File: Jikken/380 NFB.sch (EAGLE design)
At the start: 6 parts

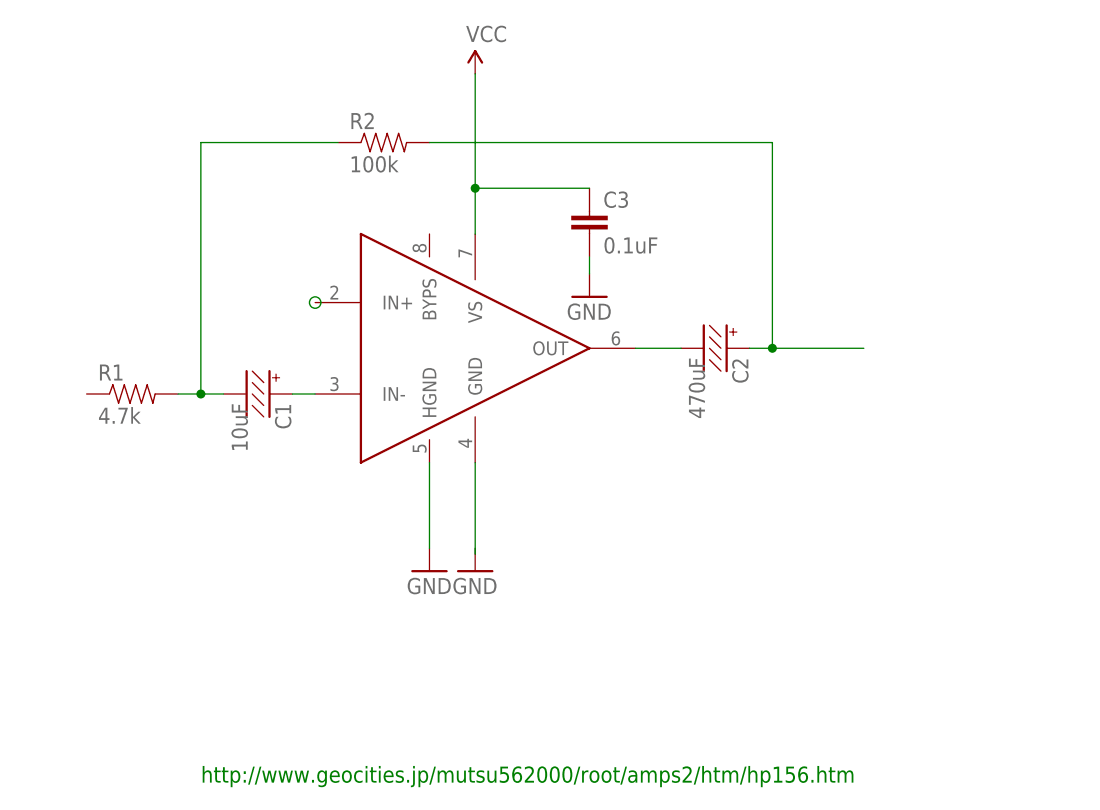
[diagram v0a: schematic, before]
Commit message: lm380
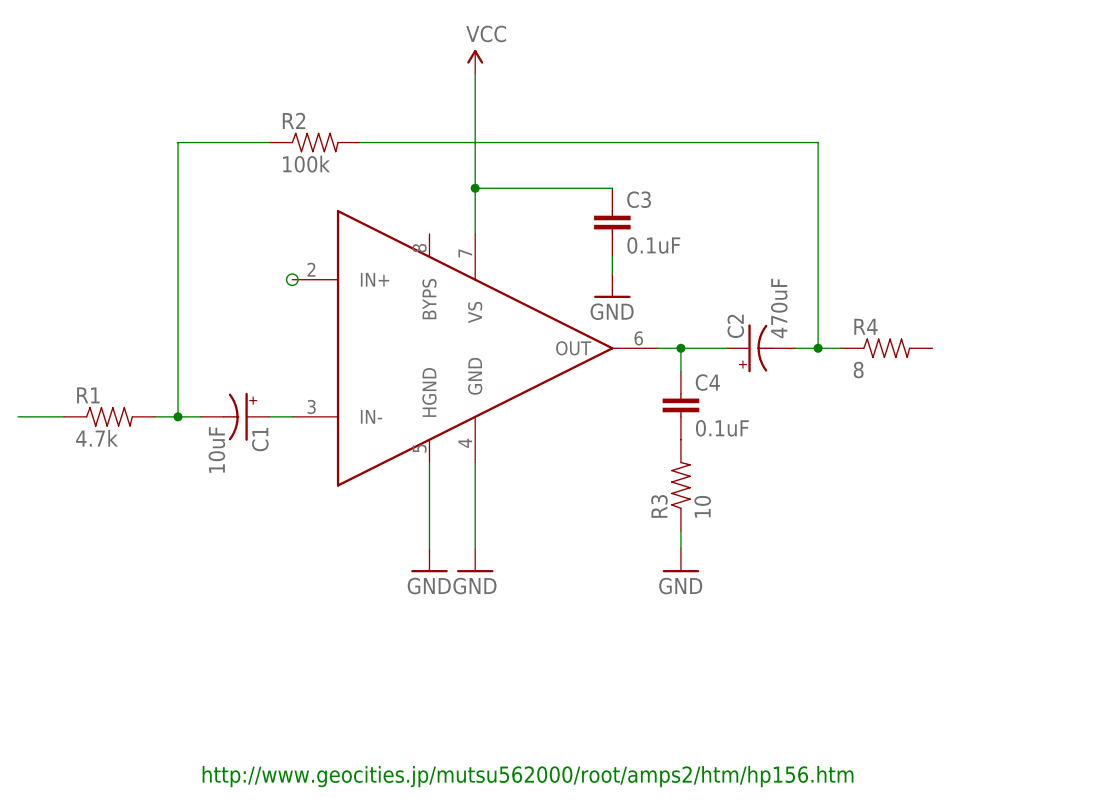
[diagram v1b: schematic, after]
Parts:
- added C4: 0.1uF, SparkFun:CAPKIT
- added R3: 10, My Library:RESISTORAXIAL-0.3
- added R4: 8, My Library:RESISTORAXIAL-0.3
- C1: device My Library:CAP_POLPTH2 -> SparkFun:CAP_POLPTH1
- C2: device My Library:CAP_POLPTH2 -> SparkFun:CAP_POLPTH4
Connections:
- removed net N$6: U$1.GND
- new net N$5: C4.2, R3.2
- new net N$7: R1.1
- net GND: now also R3.1, U$1.GND, U$1.HGND
- net N$3: now also C2.-, R4.1; no longer C2.+
- net N$4: now also C2.+, C4.1; no longer C2.-
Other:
- moved on the sheet: C3, R1, R2
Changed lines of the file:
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@@
 <part name="U$1" library="My Library" deviceset="LM380" device="N-8"/>
 <part name="R1" library="My Library" deviceset="RESISTOR" device="AXIAL-0.3" value="4.7k"/>
-<part name="C1" library="My Library" deviceset="CAP_POL" device="PTH2" value="10uF"/>
-<part name="C2" library="My Library" deviceset="CAP_POL" device="PTH2" value="470uF"/>
+<part name="C1" library="SparkFun" deviceset="CAP_POL" device="PTH1" value="10uF"/>
+<part name="C2" library="SparkFun" deviceset="CAP_POL" device="PTH4" value="470uF"/>
 <part name="R2" library="My Library" deviceset="RESISTOR" device="AXIAL-0.3" value="100k"/>
 <part name="P+1" library="SparkFun" deviceset="VCC" device=""/>
@@
 <part name="C3" library="SparkFun" deviceset="CAP" device="KIT" value="0.1uF"/>
 <part name="GND3" library="SparkFun" deviceset="GND" device=""/>
+<part name="R3" library="My Library" deviceset="RESISTOR" device="AXIAL-0.3" value="10"/>
+<part name="C4" library="SparkFun" deviceset="CAP" device="KIT" value="0.1uF"/>
+<part name="GND4" library="SparkFun" deviceset="GND" device=""/>
+<part name="R4" library="My Library" deviceset="RESISTOR" device="AXIAL-0.3" value="8"/>
 </parts>
 <sheets>
@@
 <plain>
 <text x="48.26" y="7.62" size="1.778" layer="91">http://www.geocities.jp/mutsu562000/root/amps2/htm/hp156.htm</text>
-<circle x="60.96" y="60.96" radius="0.635" width="0.1524" layer="91"/>
+<circle x="58.42" y="63.5" radius="0.635" width="0.1524" layer="91"/>
 </plain>
 <instances>
-<instance part="U$1" gate="G$1" x="76.2" y="55.88"/>
-<instance part="R1" gate="G$1" x="40.64" y="50.8"/>
-<instance part="C1" gate="G$1" x="55.88" y="50.8" rot="R270"/>
-<instance part="C2" gate="G$1" x="106.68" y="55.88" rot="R270"/>
-<instance part="R2" gate="G$1" x="68.58" y="78.74"/>
+<instance part="U$1" gate="G$1" x="78.74" y="55.88"/>
+<instance part="R1" gate="G$1" x="38.1" y="48.26"/>
+<instance part="C1" gate="G$1" x="53.34" y="48.26" rot="R270"/>
+<instance part="C2" gate="G$1" x="109.22" y="55.88" rot="R90"/>
+<instance part="R2" gate="G$1" x="60.96" y="78.74"/>
 <instance part="P+1" gate="1" x="78.74" y="86.36"/>
 <instance part="GND1" gate="1" x="78.74" y="31.115"/>
-<instance part="GND2" gate="1" x="91.44" y="61.595"/>
-<instance part="C3" gate="G$1" x="91.44" y="68.58"/>
+<instance part="GND2" gate="1" x="93.98" y="61.595"/>
+<instance part="C3" gate="G$1" x="93.98" y="68.58"/>
 <instance part="GND3" gate="1" x="73.66" y="31.115"/>
+<instance part="R3" gate="G$1" x="101.6" y="40.64" rot="R90"/>
+<instance part="C4" gate="G$1" x="101.6" y="48.26"/>
+<instance part="GND4" gate="1" x="101.6" y="31.115"/>
+<instance part="R4" gate="G$1" x="124.46" y="55.88"/>
 </instances>
 <busses>
@@
 <pinref part="C1" gate="G$1" pin="-"/>
 <pinref part="R1" gate="G$1" pin="2"/>
-<wire x1="50.8" y1="50.8" x2="48.26" y2="50.8" width="0.1524" layer="91"/>
+<wire x1="48.26" y1="48.26" x2="45.72" y2="48.26" width="0.1524" layer="91"/>
 <pinref part="R2" gate="G$1" pin="1"/>
-<wire x1="48.26" y1="50.8" x2="45.72" y2="50.8" width="0.1524" layer="91"/>
-<wire x1="63.5" y1="78.74" x2="48.26" y2="78.74" width="0.1524" layer="91"/>
-<wire x1="48.26" y1="78.74" x2="48.26" y2="50.8" width="0.1524" layer="91"/>
-<junction x="48.26" y="50.8"/>
+<wire x1="45.72" y1="48.26" x2="43.18" y2="48.26" width="0.1524" layer="91"/>
+<wire x1="55.88" y1="78.74" x2="45.72" y2="78.74" width="0.1524" layer="91"/>
+<wire x1="45.72" y1="78.74" x2="45.72" y2="48.26" width="0.1524" layer="91"/>
+<junction x="45.72" y="48.26"/>
 </segment>
 </net>
 <net name="N$3" class="0">
 <segment>
-<pinref part="C2" gate="G$1" pin="+"/>
-<wire x1="109.22" y1="55.88" x2="111.76" y2="55.88" width="0.1524" layer="91"/>
-<wire x1="111.76" y1="55.88" x2="121.92" y2="55.88" width="0.1524" layer="91"/>
-<wire x1="111.76" y1="55.88" x2="111.76" y2="78.74" width="0.1524" layer="91"/>
+<wire x1="116.84" y1="55.88" x2="119.38" y2="55.88" width="0.1524" layer="91"/>
+<wire x1="116.84" y1="55.88" x2="116.84" y2="78.74" width="0.1524" layer="91"/>
 <pinref part="R2" gate="G$1" pin="2"/>
-<wire x1="111.76" y1="78.74" x2="73.66" y2="78.74" width="0.1524" layer="91"/>
-<junction x="111.76" y="55.88"/>
-</segment>
-</net>
-<net name="N$4" class="0">
-<segment>
-<pinref part="U$1" gate="G$1" pin="OUT"/>
+<wire x1="116.84" y1="78.74" x2="66.04" y2="78.74" width="0.1524" layer="91"/>
 <pinref part="C2" gate="G$1" pin="-"/>
-<wire x1="96.52" y1="55.88" x2="101.6" y2="55.88" width="0.1524" layer="91"/>
+<wire x1="114.3" y1="55.88" x2="116.84" y2="55.88" width="0.1524" layer="91"/>
+<junction x="116.84" y="55.88"/>
+<pinref part="R4" gate="G$1" pin="1"/>
 </segment>
 </net>
@@
 <wire x1="78.74" y1="86.36" x2="78.74" y2="73.66" width="0.1524" layer="91"/>
 <wire x1="78.74" y1="73.66" x2="78.74" y2="68.58" width="0.1524" layer="91"/>
-<wire x1="78.74" y1="73.66" x2="91.44" y2="73.66" width="0.1524" layer="91"/>
+<wire x1="78.74" y1="73.66" x2="93.98" y2="73.66" width="0.1524" layer="91"/>
 <pinref part="C3" gate="G$1" pin="1"/>
 <junction x="78.74" y="73.66"/>
@@
 <wire x1="73.66" y1="43.18" x2="73.66" y2="33.655" width="0.1524" layer="91"/>
 <pinref part="GND3" gate="1" pin="GND"/>
+<pinref part="U$1" gate="G$1" pin="HGND"/>
 </segment>
 <segment>
 <pinref part="C3" gate="G$1" pin="2"/>
 <pinref part="GND2" gate="1" pin="GND"/>
-<wire x1="91.44" y1="64.135" x2="91.44" y2="66.04" width="0.1524" layer="91"/>
+<wire x1="93.98" y1="64.135" x2="93.98" y2="66.04" width="0.1524" layer="91"/>
 </segment>
-</net>
-<net name="N$6" class="0">
+<segment>
+<pinref part="R3" gate="G$1" pin="1"/>
+<pinref part="GND4" gate="1" pin="GND"/>
+<wire x1="101.6" y1="33.655" x2="101.6" y2="35.56" width="0.1524" layer="91"/>
+</segment>
 <segment>
 <pinref part="U$1" gate="G$1" pin="GND"/>
-<wire x1="78.74" y1="43.18" x2="78.74" y2="33.02" width="0.1524" layer="91"/>
+<wire x1="78.74" y1="43.18" x2="78.74" y2="33.655" width="0.1524" layer="91"/>
+<pinref part="GND1" gate="1" pin="GND"/>
 </segment>
 </net>
@@
 <pinref part="C1" gate="G$1" pin="+"/>
 <pinref part="U$1" gate="G$1" pin="IN-"/>
-<wire x1="58.42" y1="50.8" x2="60.96" y2="50.8" width="0.1524" layer="91"/>
+<wire x1="55.88" y1="48.26" x2="58.42" y2="48.26" width="0.1524" layer="91"/>
 </segment>
 </net>
+<net name="N$4" class="0">
+<segment>
+<pinref part="U$1" gate="G$1" pin="OUT"/>
+<pinref part="C2" gate="G$1" pin="+"/>
+<wire x1="99.06" y1="55.88" x2="101.6" y2="55.88" width="0.1524" layer="91"/>
+<pinref part="C4" gate="G$1" pin="1"/>
+<wire x1="101.6" y1="55.88" x2="106.68" y2="55.88" width="0.1524" layer="91"/>
+<wire x1="101.6" y1="55.88" x2="101.6" y2="53.34" width="0.1524" layer="91"/>
+<junction x="101.6" y="55.88"/>
+</segment>
+</net>
+<net name="N$5" class="0">
+<segment>
+<pinref part="C4" gate="G$1" pin="2"/>
+<pinref part="R3" gate="G$1" pin="2"/>
+</segment>
+</net>
+<net name="N$7" class="0">
+<segment>
+<pinref part="R1" gate="G$1" pin="1"/>
+<wire x1="33.02" y1="48.26" x2="27.94" y2="48.26" width="0.1524" layer="91"/>
+</segment>
+</net>
